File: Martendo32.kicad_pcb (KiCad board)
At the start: 2 copper layers, 75.2 x 98.5 mm, 110 parts, among them CN2 ZX-MX1.25-2PWT, J1 AudioJack4_SwitchTR1, J2 Conn_01x03, J3 Conn_01x18_Socket, J4 USB-C, Q1 NPN, Q2 AO3401A, SW1 SK-3296S-01-L3, U3 TP4056, U4 NS4168, U5 TPS61040DBV, U6 AP2112K-3.3

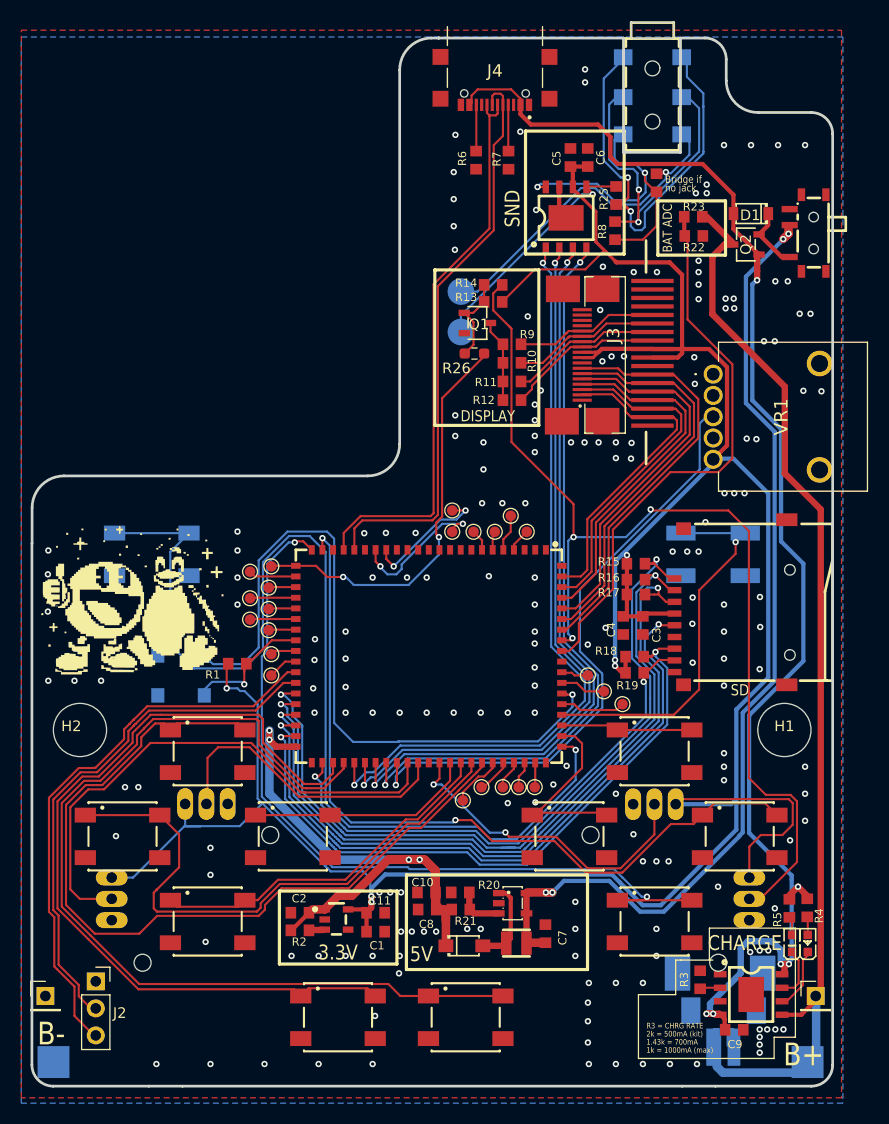
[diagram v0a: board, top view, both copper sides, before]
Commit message: Add files via upload
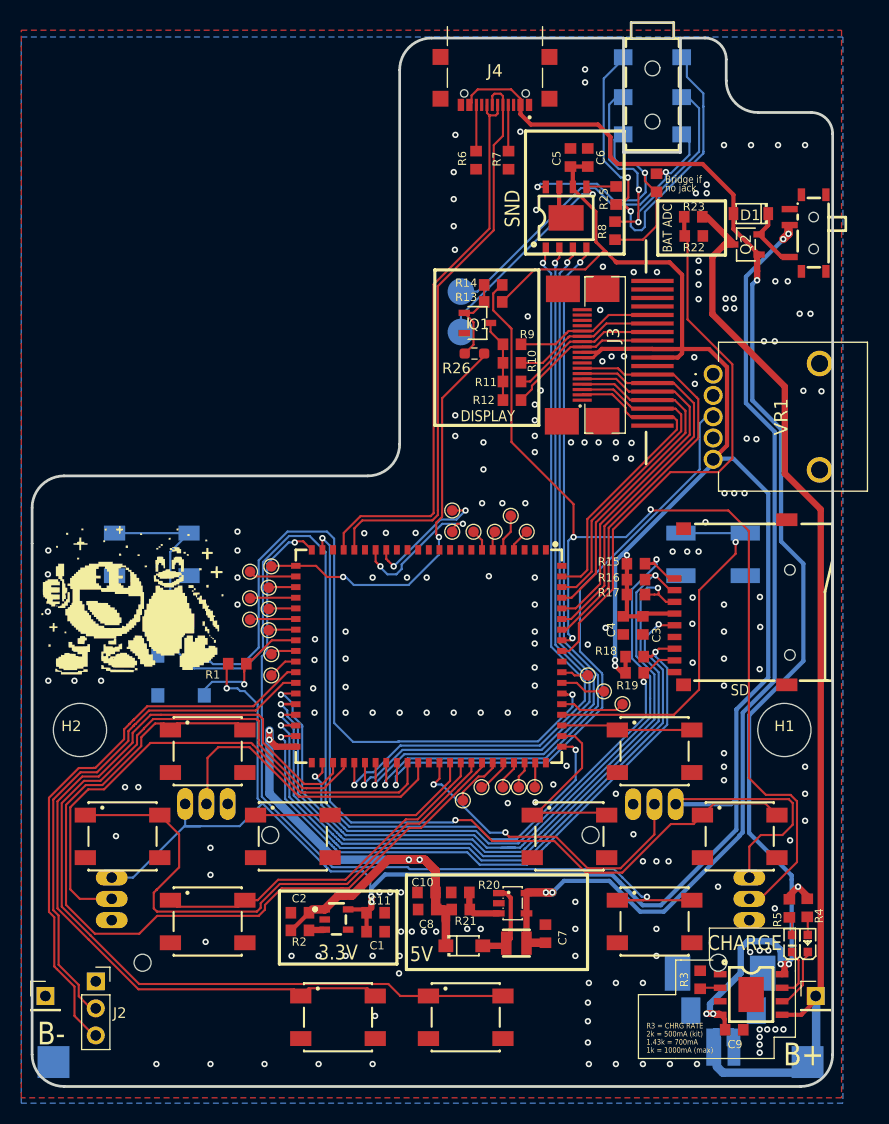
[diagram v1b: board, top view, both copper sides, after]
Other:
- outline, holes or cut-outs redrawn
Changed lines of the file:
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@@
 		)
 		(embedded_fonts no)
+		(model "Y:/KiCAD/3D/687118183722_Download_STP_687118183722_rev1.stp"
+			(offset
+				(xyz 0 0 0)
+			)
+			(scale
+				(xyz 1 1 1)
+			)
+			(rotate
+				(xyz 0 0 0)
+			)
+		)
 	)
 	(footprint "KiCad_GB300-P4-SingleSided_SMT_V2:0603"
@@
 		(layer "F.SilkS")
 	)
-	(gr_line
-		(start 46.59 149.578)
-		(end 46.59 100.578)
-		(stroke
-			(width 0.254)
-			(type default)
-		)
-		(layer "Edge.Cuts")
-	)
 	(gr_arc
 		(start 46.606 97.2276)
@@
 		(layer "Edge.Cuts")
 	)
-	(gr_arc
-		(start 48.59 151.578)
-		(mid 47.175786 150.992214)
-		(end 46.59 149.578)
+	(gr_line
+		(start 46.606 148.605)
+		(end 46.606 100.578)
 		(stroke
 			(width 0.254)
-			(type default)
+			(type solid)
 		)
 		(layer "Edge.Cuts")
 	)
-	(gr_line
-		(start 48.59 151.578)
-		(end 57.59 151.578)
+	(gr_arc
+		(start 49.606 151.605)
+		(mid 47.48468 150.72632)
+		(end 46.606 148.605)
 		(stroke
 			(width 0.254)
@@
 	)
 	(gr_line
-		(start 57.59 151.578)
-		(end 60.74 151.578)
+		(start 49.606 151.605)
+		(end 118.84 151.605)
 		(stroke
 			(width 0.254)
@@
 	)
 	(gr_line
-		(start 60.74 151.578)
-		(end 107.69 151.578)
-		(stroke
-			(width 0.254)
-			(type default)
-		)
-		(layer "Edge.Cuts")
-	)
-	(gr_line
 		(start 78.15 94.2276)
 		(end 49.606 94.2276)
@@
 	)
 	(gr_line
-		(start 84.79 53.078)
-		(end 84.8375 53.078)
-		(stroke
-			(width 0.254)
-			(type solid)
-		)
-		(layer "Edge.Cuts")
-	)
-	(gr_line
-		(start 84.8375 53.078)
-		(end 84.15 53.078)
-		(stroke
-			(width 0.254)
-			(type solid)
-		)
-		(layer "Edge.Cuts")
-	)
-	(gr_line
 		(start 102.19 53.078)
-		(end 84.8375 53.078)
+		(end 84.15 53.078)
 		(stroke
 			(width 0.254)
@@
 		(layer "Edge.Cuts")
 	)
-	(gr_line
-		(start 107.69 151.578)
-		(end 110.84 151.578)
-		(stroke
-			(width 0.254)
-			(type solid)
-		)
-		(layer "Edge.Cuts")
-	)
 	(gr_arc
 		(start 109.84 53.078)
@@
 		(layer "Edge.Cuts")
 	)
-	(gr_line
-		(start 119.84 151.578)
-		(end 110.84 151.578)
-		(stroke
-			(width 0.254)
-			(type default)
-		)
-		(layer "Edge.Cuts")
-	)
 	(gr_arc
-		(start 121.84 149.578)
-		(mid 121.254214 150.992214)
-		(end 119.84 151.578)
+		(start 121.84 148.605)
+		(mid 120.96132 150.72632)
+		(end 118.84 151.605)
 		(stroke
 			(width 0.254)
@@
 	)
 	(gr_line
-		(start 121.84 149.578)
+		(start 121.84 148.605)
 		(end 121.84 62.078)
 		(stroke
@@
 	)
 	(segment
-		(start 71.39 115.678)
-		(end 70.39 115.678)
+		(start 105.19 103.578)
+		(end 104.607 103.578)
 		(width 0.2)
 		(layer "F.Cu")
@@
 	)
 	(segment
-		(start 105.19 103.578)
-		(end 104.607 103.578)
-		(width 0.2)
+		(start 71.39 115.678)
+		(end 69.99 115.678)
+		(width 0.254)
 		(layer "F.Cu")
 		(net "/SD_CD")
@@
 	)
 	(segment
-		(start 71.591 117.9934)
-		(end 71.591 124.079)
-		(width 0.2)
-		(layer "B.Cu")
-		(net "/SD_CD")
-	)
-	(segment
 		(start 105.19 103.578)
 		(end 105.1424 103.6256)
@@
 	)
 	(segment
+		(start 69.99 115.678)
+		(end 69.99 115.6812)
+		(width 0.2)
+		(layer "B.Cu")
+		(net "/SD_CD")
+	)
+	(segment
 		(start 105.1424 103.6256)
 		(end 104.9424 103.6256)
@@
 	)
 	(segment
-		(start 70.19 115.678)
-		(end 70.59 116.078)
+		(start 71.59 117.833115)
+		(end 71.59 117.9924)
 		(width 0.2)
 		(layer "B.Cu")
@@
 	)
 	(segment
-		(start 69.99 115.678)
-		(end 70.19 115.678)
+		(start 103.391 111.179)
+		(end 105.091 112.879)
 		(width 0.2)
 		(layer "B.Cu")
@@
 	)
 	(segment
-		(start 103.391 111.179)
-		(end 105.091 112.879)
+		(start 71.591 124.079)
+		(end 73.99 126.478)
 		(width 0.2)
 		(layer "B.Cu")
@@
 	)
 	(segment
-		(start 70.59 116.078)
-		(end 70.59 116.833114)
+		(start 69.99 115.6812)
+		(end 70.59 116.2812)
 		(width 0.2)
 		(layer "B.Cu")
@@
 	)
 	(segment
-		(start 71.591 124.079)
-		(end 73.99 126.478)
+		(start 92.969271 129.2288)
+		(end 92.88047 129.3176)
 		(width 0.2)
 		(layer "B.Cu")
@@
 	)
 	(segment
-		(start 92.969271 129.2288)
-		(end 92.88047 129.3176)
+		(start 75.61323 128.098401)
+		(end 75.467229 127.9524)
 		(width 0.2)
 		(layer "B.Cu")
@@
 	)
 	(segment
-		(start 75.61323 128.098401)
-		(end 75.467229 127.9524)
+		(start 70.59 116.833114)
+		(end 71.59 117.833115)
 		(width 0.2)
 		(layer "B.Cu")
@@
 	)
 	(segment
-		(start 71.59 117.833115)
-		(end 71.59 117.9924)
+		(start 71.591 117.9934)
+		(end 71.591 124.079)
 		(width 0.2)
 		(layer "B.Cu")
@@
 	)
 	(segment
-		(start 70.59 116.833114)
-		(end 71.59 117.833115)
+		(start 70.59 116.2812)
+		(end 70.59 116.833114)
 		(width 0.2)
 		(layer "B.Cu")
